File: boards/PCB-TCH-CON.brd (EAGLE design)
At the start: 50 x 23 mm, 13 parts

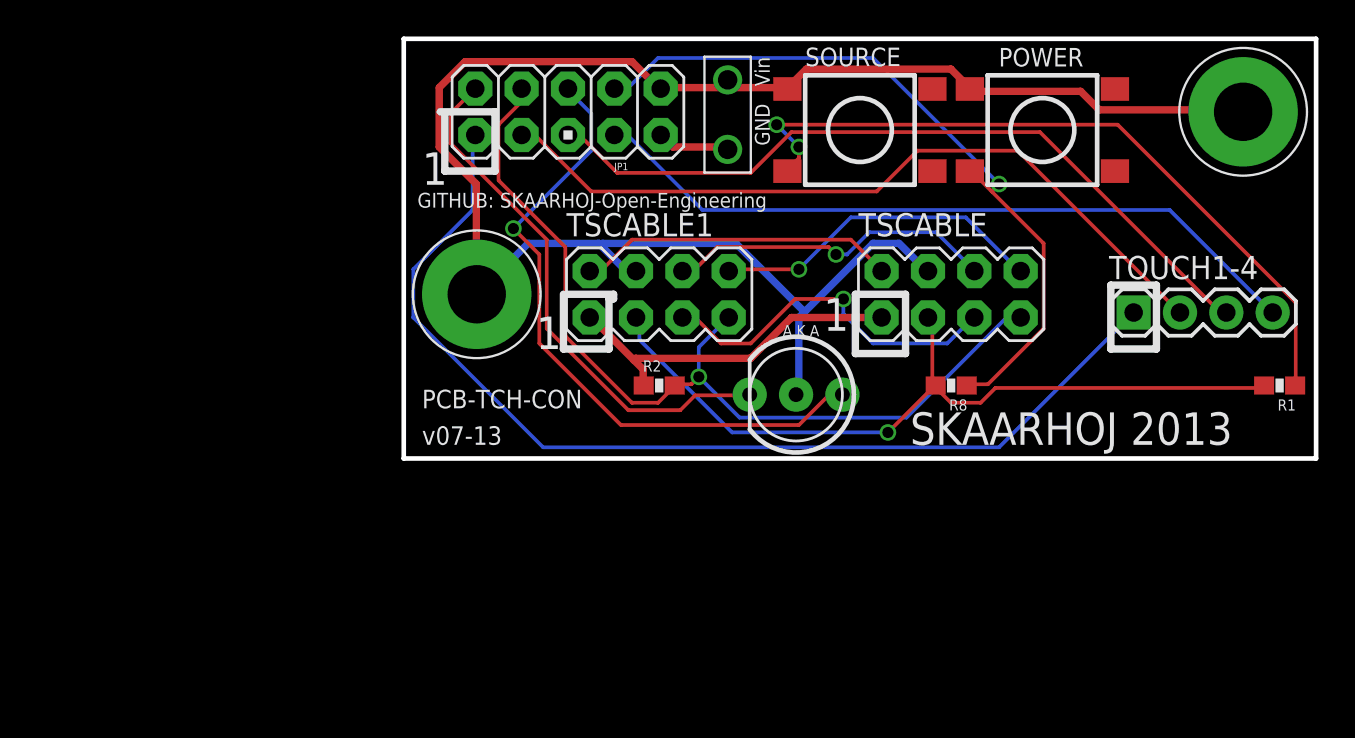
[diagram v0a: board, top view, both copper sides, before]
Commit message: put all the downloaded files into directories
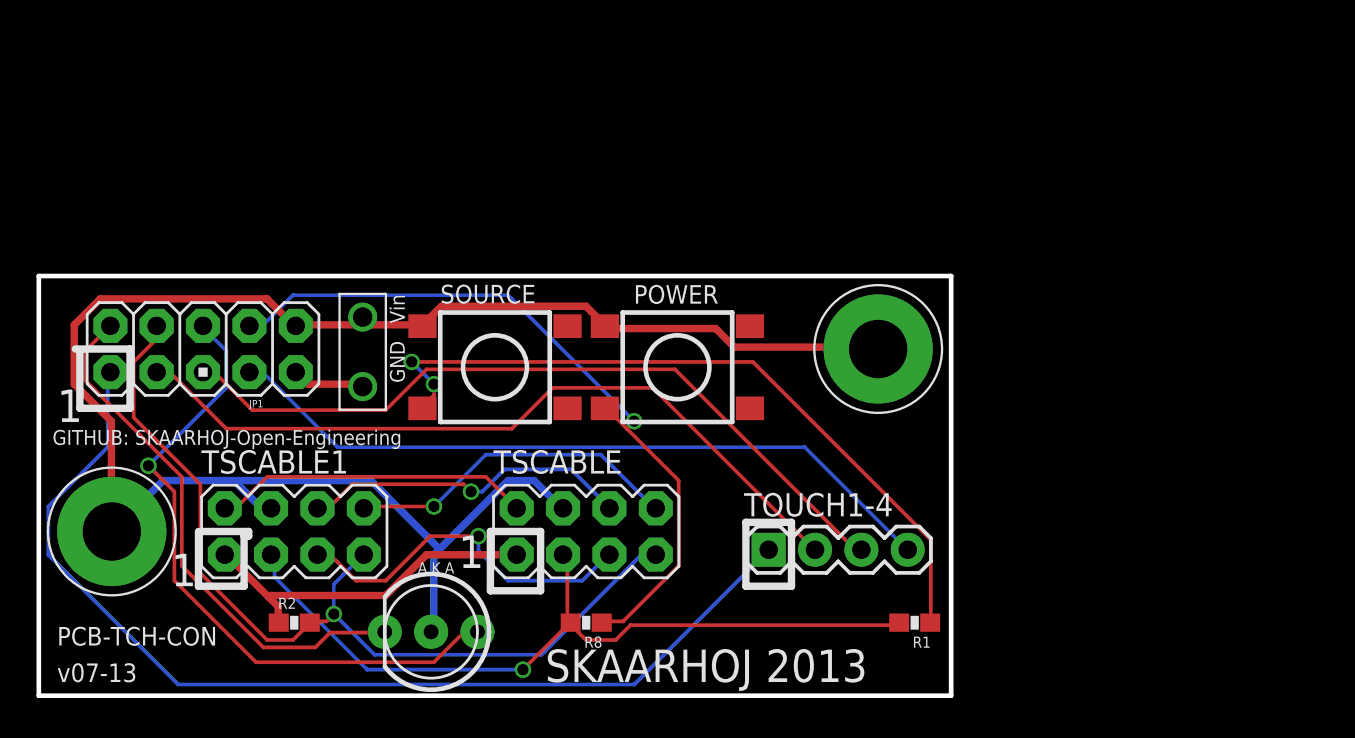
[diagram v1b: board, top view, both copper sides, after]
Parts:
- moved JP1 23.9 mm to (9.00, 19.0)
- moved ON 23.9 mm to (35.0, 18.0)
- moved R1 23.9 mm to (48.0, 4.00)
- moved R2 23.9 mm to (14.0, 4.00)
- moved R8 23.9 mm to (30.0, 4.00)
- moved SRC 23.9 mm to (25.0, 18.0)
- moved TOUCH1-4 23.9 mm to (40.0, 8.00)
- moved TSCABLE 23.9 mm to (30.0, 9.00)
- moved TSCABLE1 23.9 mm to (14.0, 9.00)
- moved U$15 23.9 mm to (4.00, 9.00)
- moved U$2 23.9 mm to (21.5, 3.50)
- moved U$20 23.9 mm to (46.0, 19.0)
- moved VIN1 23.9 mm to (17.8, 20.8)
